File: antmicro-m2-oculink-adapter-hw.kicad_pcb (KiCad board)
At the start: 4 copper layers, 22 x 80 mm, 14 parts, among them J1 PCB-Edge_M.2_Key-M, J2 OCuLink_x4_Amphenol_G14A42121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

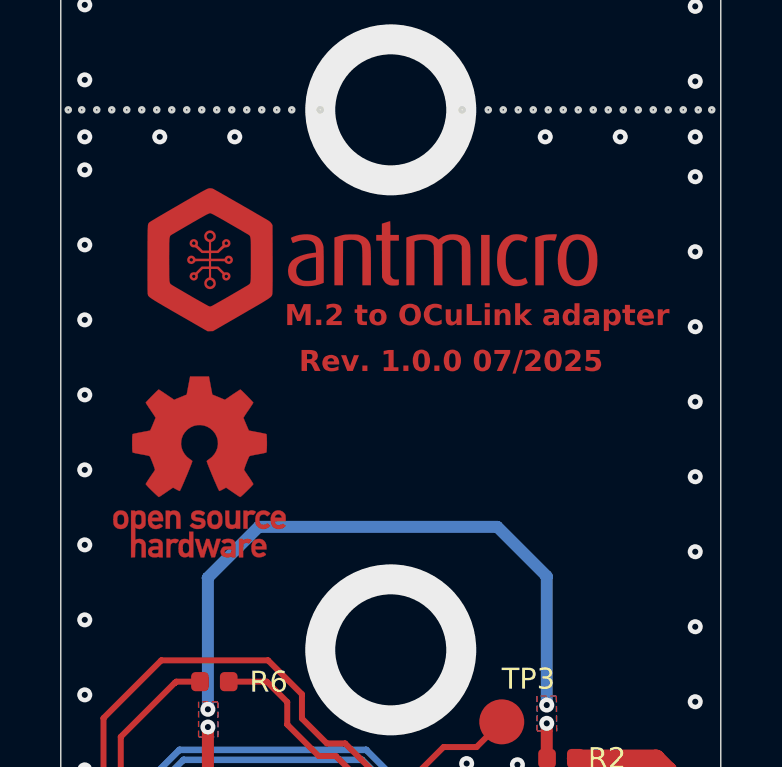
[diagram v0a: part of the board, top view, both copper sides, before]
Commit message: [#80747] Fix DRC
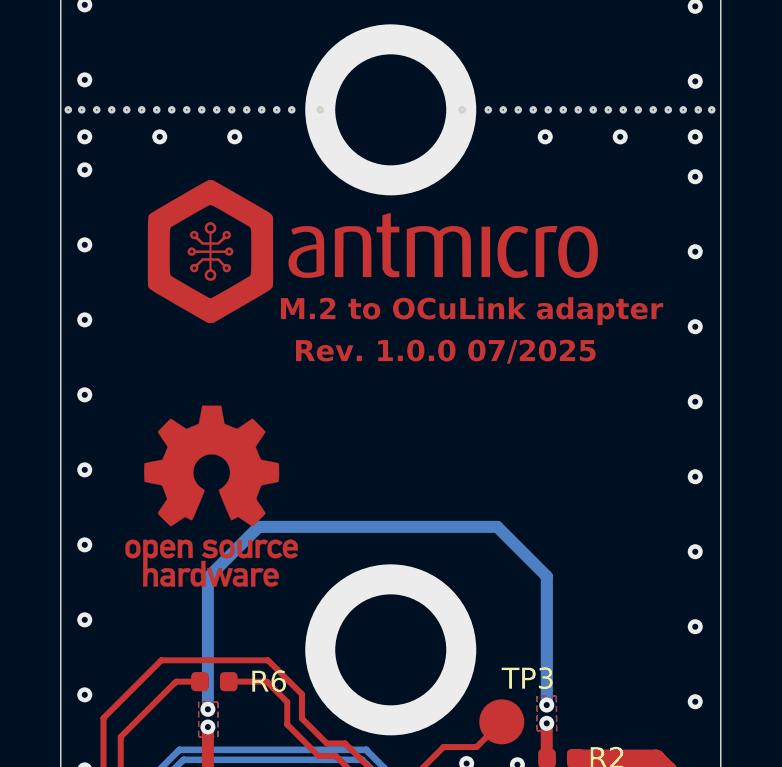
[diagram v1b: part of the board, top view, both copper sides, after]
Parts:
- moved REF** 1.06 mm to (140.2, 83.5) (x2)
- moved REF** 0.28 mm to (146.0, 75.4)
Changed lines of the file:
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@@
 	(footprint "antmicro-footprints:antmicro-logo_scaled_15mm"
 		(layer "F.Cu")
-		(at 145.99 75.67)
+		(at 146.005 75.395)
 		(property "Reference" "REF**"
 			(at 0.1 -3 0)
@@
 	(footprint "antmicro-footprints:OSHW-Logo_5.7x6mm_Mask"
 		(layer "F.Cu")
-		(at 139.77 82.5)
+		(at 140.175 83.475)
 		(descr "Open Source Hardware Logo")
 		(tags "Logo OSHW")
@@
 	(footprint "antmicro-footprints:OSHW-Logo_5.7x6mm_Copper"
 		(layer "F.Cu")
-		(at 139.77 82.5)
+		(at 140.175 83.475)
 		(descr "Open Source Hardware Logo")
 		(tags "Logo OSHW")
@@
 	)
 	(gr_text "${TITLE}"
-		(at 148.86 77.45 0)
+		(at 148.65 77.25 0)
 		(layer "F.Cu")
 		(effects
@@
 	)
 	(gr_text "Rev. 1.0.0 07/2025\n"
-		(at 148.16 78.98 0)
+		(at 147.975 78.65 0)
 		(layer "F.Cu")
 		(effects
@@
 	)
 	(gr_text "${TITLE}"
-		(at 148.86 77.45 0)
+		(at 148.65 77.25 0)
 		(layer "F.Mask")
 		(effects
@@
 	)
 	(gr_text "Rev. 1.0.0 07/2025\n"
-		(at 148.16 78.98 0)
+		(at 147.975 78.65 0)
 		(layer "F.Mask")
 		(effects
